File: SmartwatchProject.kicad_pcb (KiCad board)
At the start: 2 copper layers, 7 parts, among them J1 USB_B_Micro, U1 ESP32-S3-WROOM-1, U2 DS3231M, U6 MAX98357A, U8 AMS1117-3.3, U9 MCP73831-2-MC

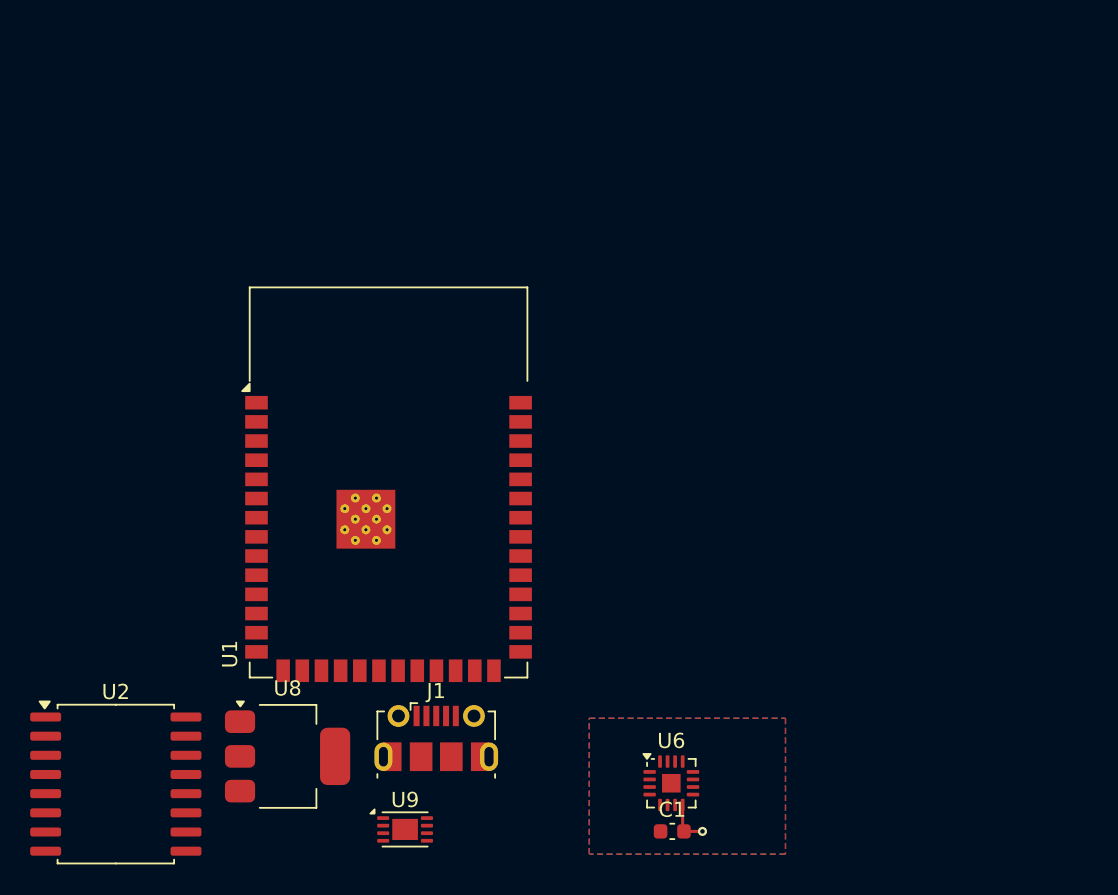
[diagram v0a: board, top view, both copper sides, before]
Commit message: PCB Draft
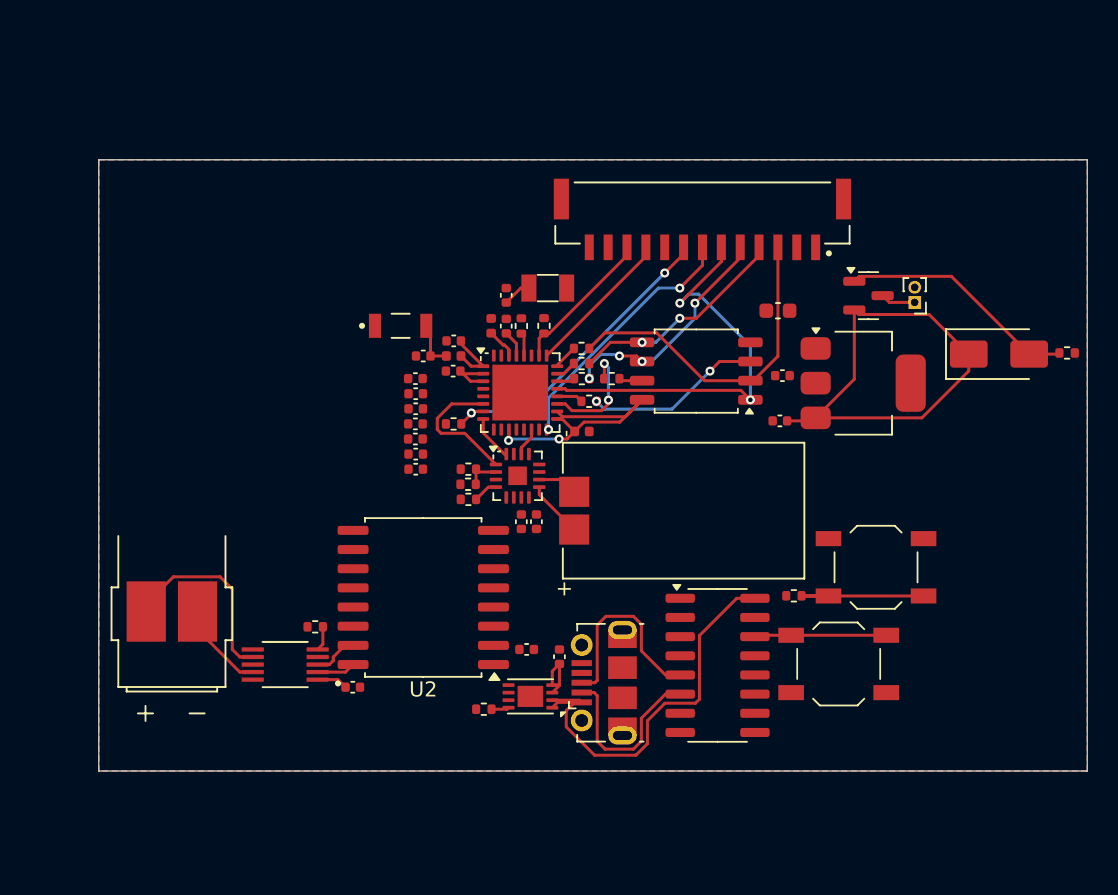
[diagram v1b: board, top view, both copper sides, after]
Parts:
- removed U9: MCP73831-2-MC, Package_DFN_QFN:DFN-8-1EP_3x2mm_P0.5mm_EP1.7x1.4mm
- added AE1: AMCA31-2R450G-S1F-T3, Imports_Global:XDCR_AMCA31-2R450G-S1F-T3, F.Cu at (143.5, 82.0)
- added B1: HD-EMB1408-SC, HD-EMB1408-SC:MOTOR_HD-EMB1408-SC, F.Cu at (128.3, 100.9)
- added BT1: Battery_Cell, Connector_PinHeader_1.00mm:PinHeader_1x02_P1.00mm_Vertical, F.Cu at (177.6, 80.5)
- added C10: TBD, Capacitor_SMD:C_0402_1005Metric, F.Cu at (147.0, 83.0)
- added C11: TBD, Capacitor_SMD:C_0402_1005Metric, F.Cu at (145.0, 84.0)
- added C12: 0.1uF, Capacitor_SMD:C_0402_1005Metric, F.Cu at (144.5, 85.5)
- added C13: 1uF, Capacitor_SMD:C_0402_1005Metric, F.Cu at (147.0, 85.0)
- added C14: 10uF, Capacitor_SMD:C_0402_1005Metric, F.Cu at (144.5, 86.5)
- added C15: 0.1uF, Capacitor_SMD:C_0402_1005Metric, F.Cu at (144.5, 87.5)
- added C16: 0.1uF, Capacitor_SMD:C_0402_1005Metric, F.Cu at (144.5, 88.5)
- added C17: 1uF, Capacitor_SMD:C_0402_1005Metric, F.Cu at (144.5, 89.5)
- added C18: 1uF, Capacitor_SMD:C_0402_1005Metric, F.Cu at (144.5, 90.5)
- added C19: 10nF, Capacitor_SMD:C_0402_1005Metric, F.Cu at (144.5, 91.5)
- added C2: 10µF, Capacitor_SMD:C_0402_1005Metric, F.Cu at (140.3, 105.9)
- added C20: TBD, Capacitor_SMD:C_0402_1005Metric, F.Cu at (150.5, 82.0)
- added C21: TBD, Capacitor_SMD:C_0402_1005Metric, F.Cu at (150.5, 80.0)
- added C3: 10uF, Capacitor_SMD:C_0402_1005Metric, F.Cu at (168.6, 88.3)
- added C4: 22uF, Capacitor_SMD:C_0402_1005Metric, F.Cu at (168.8, 85.3)
- added C5: 1uF, Capacitor_SMD:C_0402_1005Metric, F.Cu at (152.5, 95.0)
- added C6: 0.1uF, Capacitor_SMD:C_0402_1005Metric, F.Cu at (151.5, 95.0)
- added C7: 10uF, Capacitor_SMD:C_0402_1005Metric, F.Cu at (151.8, 103.4)
- added C8: 4.7uF, Capacitor_SMD:C_0402_1005Metric, F.Cu at (154.0, 103.9)
- added D1: SS210, Diode_SMD:D_SMA, F.Cu at (183.1, 83.9)
- added J2: SM13B-GHS-TB_LF__SN_, Imports_Global:JST_SM13B-GHS-TB_LF__SN_, F.Cu at (163.5, 73.6)
- added L1: 0.2nH, Inductor_SMD:L_0402_1005Metric, F.Cu at (147.0, 84.0)
- added L2: 0.2nH, Inductor_SMD:L_0402_1005Metric, F.Cu at (155.5, 89.0)
- added L3: TBD, Inductor_SMD:L_0402_1005Metric, F.Cu at (149.5, 82.0)
- added LS1: CMS-16098A-SP, Imports_Global:CUI_CMS-16098A-SP, F.Cu at (162.2, 94.2)
- added Q1: AO3401A, Package_TO_SOT_SMD:SOT-23, F.Cu at (174.5, 80.0)
- added R1: 4.7k, Resistor_SMD:R_0402_1005Metric, F.Cu at (153.0, 82.0)
- added R10: 0, Resistor_SMD:R_0402_1005Metric, F.Cu at (156.0, 87.0)
- added R11: 0, Resistor_SMD:R_0402_1005Metric, F.Cu at (155.5, 85.5)
- added R12: 0, Resistor_SMD:R_0402_1005Metric, F.Cu at (155.5, 84.5)
- added R13: 0, Resistor_SMD:R_0402_1005Metric, F.Cu at (155.5, 83.5)
- added R14: 499, Resistor_SMD:R_0402_1005Metric, F.Cu at (151.5, 82.0)
- added R15: 4.7k, Resistor_SMD:R_0402_1005Metric, F.Cu at (137.8, 101.9)
- added R16: 4.7k, Resistor_SMD:R_0402_1005Metric, F.Cu at (187.7, 83.8)
- added R3: 10k, Resistor_SMD:R_0402_1005Metric, F.Cu at (147.0, 88.5)
- added R4: 10k, Resistor_SMD:R_0402_1005Metric, F.Cu at (169.6, 99.9)
- added R5: 2k, Resistor_SMD:R_0402_1005Metric, F.Cu at (149.0, 107.4)
- added R6: 0, Resistor_SMD:R_0402_1005Metric, F.Cu at (148.0, 91.5)
- added R7: 0, Resistor_SMD:R_0402_1005Metric, F.Cu at (148.0, 92.5)
- added R8: 1M, Resistor_SMD:R_0402_1005Metric, F.Cu at (148.0, 93.5)
- added R9: 0, Resistor_SMD:R_0402_1005Metric, F.Cu at (157.5, 85.5)
- added SW1: SW_Push, Button_Switch_SMD:SW_SPST_TL3342, F.Cu at (172.5, 104.4)
- added SW2: SW_Push, Button_Switch_SMD:SW_SPST_TL3342, F.Cu at (175.0, 98.0)
- added U3: MCP73831-2-MC, Package_DFN_QFN:DFN-8-1EP_3x2mm_P0.5mm_EP1.7x1.4mm, F.Cu at (152.1, 106.6)
- added U4: DRV2605LDGSR, DRV2605LDGSR:SOP50P490X110-10N, F.Cu at (135.8, 104.4)
- added U5: ESP32-C3, Package_DFN_QFN:QFN-32-1EP_5x5mm_P0.5mm_EP3.7x3.7mm, F.Cu at (151.4, 86.4)
- added U7: W25Q32JVSS, Package_SO:SOIC-8_5.3x5.3mm_P1.27mm, F.Cu at (163.1, 85.0)
- added Y1: 40MHz, Crystal:Crystal_SMD_3215-2Pin_3.2x1.5mm, F.Cu at (153.2, 79.5)
- U1: value ESP32-S3-WROOM-1 -> CH340C; footprint RF_Module:ESP32-S3-WROOM-1 -> Package_SO:SOIC-16_3.9x9.9mm_P1.27mm
- moved U8 45.5 mm to (174.2, 85.8)
- moved C1 35.2 mm to (168.5, 81.0)
- moved U1 25.0 mm to (164.5, 104.5)
- moved U2 23.8 mm to (145.0, 100.0), turned to 180 degrees
- moved U6 22.8 mm to (151.2, 91.9)
- moved J1 11.7 mm to (157.0, 105.7), turned to 90 degrees
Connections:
- U1 pad 13: /D- -> unconnected-(U1-~{DTR}-Pad13)
- U1 pad 14: /D+ -> /RST
- U1 pad 15: /IO3 -> unconnected-(U1-R232-Pad15)
- U1 pad 16: unconnected-(U1-IO46-Pad16) -> /USB5V
- U1 pad 2: +3.3V -> /TXD
- U1 pad 3: unconnected-(U1-EN-Pad3) -> /RXD
- U1 pad 4: /IRQ -> +3.3V
- U1 pad 5: /GAIN -> /D+
- U1 pad 6: /SDA -> /D-
- U1 pad 7: /SCL -> unconnected-(U1-NC-Pad7)
- U1 pad 8: /BCLK -> unconnected-(U1-NC-Pad8)
- U1 pad 9: /LRCLK -> unconnected-(U1-~{CTS}-Pad9)
- U2 pad 3: /INT -> unconnected-(U2-~{INT}/SQW-Pad3)
- U2 pad 4: /RST1 -> unconnected-(U2-~{RST}-Pad4)
- U6 pad 17: unconnected-(U6-PAD-Pad17) -> GND
- U6 pad 2: /GAIN -> Net-(U6-GAIN_SLOT)
- U6 pad 4: /SD MODE -> Net-(U6-~{SD_MODE})
- U8 pad 3: /USB5V -> Net-(D1-K)
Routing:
- net /USB5V: track 0.00 -> 43.3 mm
- net Net-(D1-K): track 0.00 -> 31.5 mm
- net /RST: track 0.00 -> 29.4 mm, vias 0 -> 2
- net /CS: track 0.00 -> 27.9 mm, vias 0 -> 2
- net /MISO: track 0.00 -> 22.1 mm
- net TBD: track 0.00 -> 18.4 mm, vias 0 -> 2
- net /DC: track 0.00 -> 17.1 mm, vias 0 -> 2
- net /SCK: track 0.00 -> 15.5 mm, vias 0 -> 4
- net /MOSI: track 0.00 -> 14.8 mm, vias 0 -> 2
- net /D+: track 0.00 -> 13.1 mm
- net /SDA: track 0.00 -> 12.9 mm
- net Net-(U4-OUT+): track 0.00 -> 12.8 mm
- net /SCL: track 0.00 -> 12.3 mm
- net /D-: track 0.00 -> 12.3 mm
- net /LSPIWP: track 0.00 -> 11.8 mm, vias 0 -> 2
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- added copper zone on F.Cu, net +3.3V
- added copper zone on B.Cu, net GND
- removed copper zone on B.Cu, net +3.3V
- removed copper zone on F.Cu, net GND
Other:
- board outline added: 65.5 x 40.5 mm

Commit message: Schematic Draft
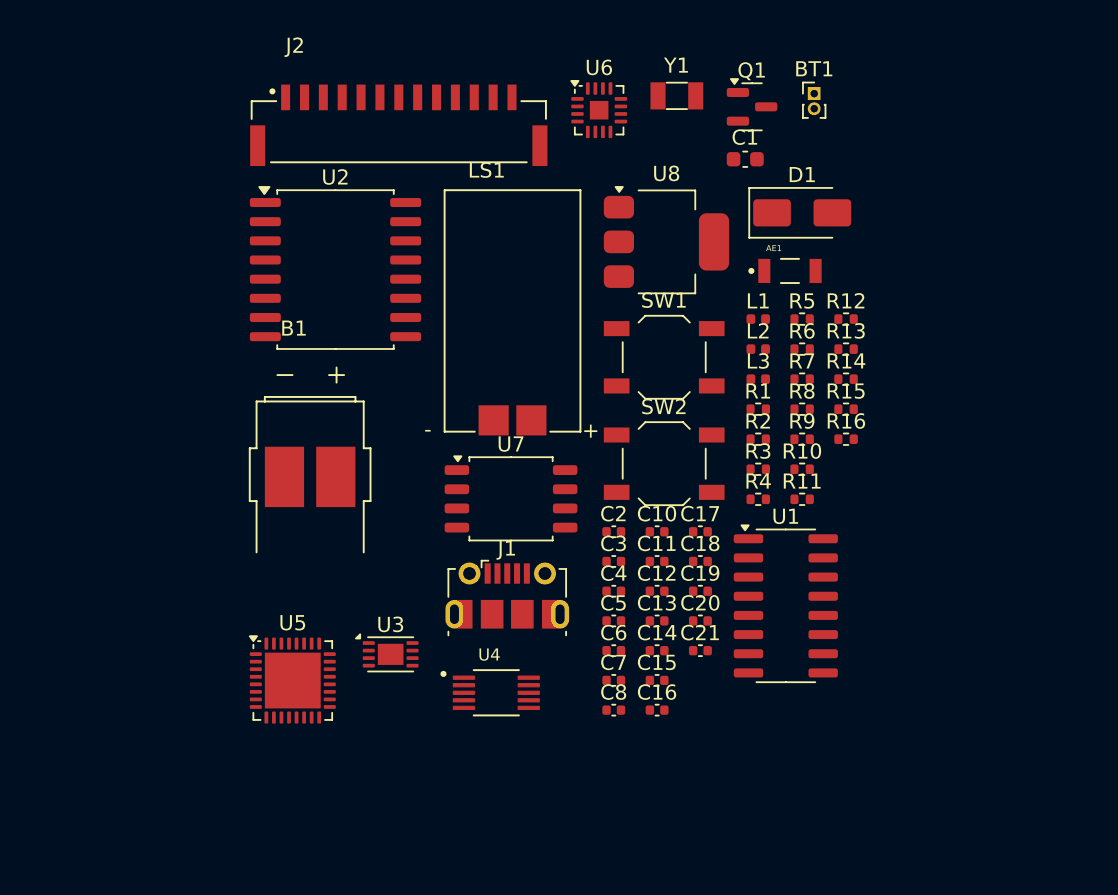
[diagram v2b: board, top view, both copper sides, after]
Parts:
- added R2: 4.7k, Resistor_SMD:R_0402_1005Metric, F.Cu at (167.2, 89.5)
- moved R15 38.0 mm to (173.0, 87.5)
- moved R5 33.4 mm to (170.1, 81.6), turned to 0 degrees
- moved C21 26.8 mm to (163.4, 103.5), turned to 0 degrees
- moved AE1 26.1 mm to (169.3, 78.4)
- moved C16 24.8 mm to (160.5, 107.5)
- moved U6 24.8 mm to (156.7, 67.7)
- moved U5 24.3 mm to (136.4, 105.5)
- moved C15 24.1 mm to (160.5, 105.5)
- moved R6 23.5 mm to (170.1, 83.5)
- moved C20 23.4 mm to (163.4, 101.6), turned to 0 degrees
- moved SW1 23.4 mm to (161.0, 84.1), turned to 0 degrees
- moved C14 23.4 mm to (160.5, 103.5)
- moved R7 23.2 mm to (170.1, 85.5)
- moved R8 22.9 mm to (170.1, 87.5)
- moved U2 22.5 mm to (139.2, 78.3), turned to 0 degrees
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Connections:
- J2 pad 6: /CS -> /Display_CS
- U5 pad 14: /LRCLK -> /SDA
- U5 pad 15: unconnected-(U5-GPIO9-Pad15) -> /SCL
- U5 pad 16: /DC -> /DIN
- U5 pad 25: /SDA -> /Display_CS
- U5 pad 26: /SCL -> /DC
- U5 pad 6: /DIN -> /BCLK
- U5 pad 8: /BCLK -> /LRCLK
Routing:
- net /USB5V: track 43.3 -> 0.00 mm
- net Net-(D1-K): track 31.5 -> 0.00 mm
- net /RST: track 29.4 -> 0.00 mm, vias 2 -> 0
- net /CS: track 27.9 -> 0.00 mm, vias 2 -> 0
- net /MISO: track 22.1 -> 0.00 mm
- net TBD: track 18.4 -> 0.00 mm, vias 2 -> 0
- net /DC: track 17.1 -> 0.00 mm, vias 2 -> 0
- net /SCK: track 15.5 -> 0.00 mm, vias 4 -> 0
- net /MOSI: track 14.8 -> 0.00 mm, vias 2 -> 0
- net /D+: track 13.1 -> 0.00 mm
- net /SDA: track 12.9 -> 0.00 mm
- net Net-(U4-OUT+): track 12.8 -> 0.00 mm
- net /SCL: track 12.3 -> 0.00 mm
- net /D-: track 12.3 -> 0.00 mm
- net /LSPIWP: track 11.8 -> 0.00 mm, vias 2 -> 0
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- removed copper zone on F.Cu, net +3.3V
- removed copper zone on B.Cu, net GND
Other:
- board outline removed
